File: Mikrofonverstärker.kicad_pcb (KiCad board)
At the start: 2 copper layers, 50.5 x 37.3 mm, 60 parts, among them J1 Screw_Terminal_01x02, J3 Screw_Terminal_01x02, J4 Screw_Terminal_01x03, J5 USB_C_Receptacle_USB2.0_14P, U1 CM108B, U2 THAT151xx08, U3 NMA0515SC

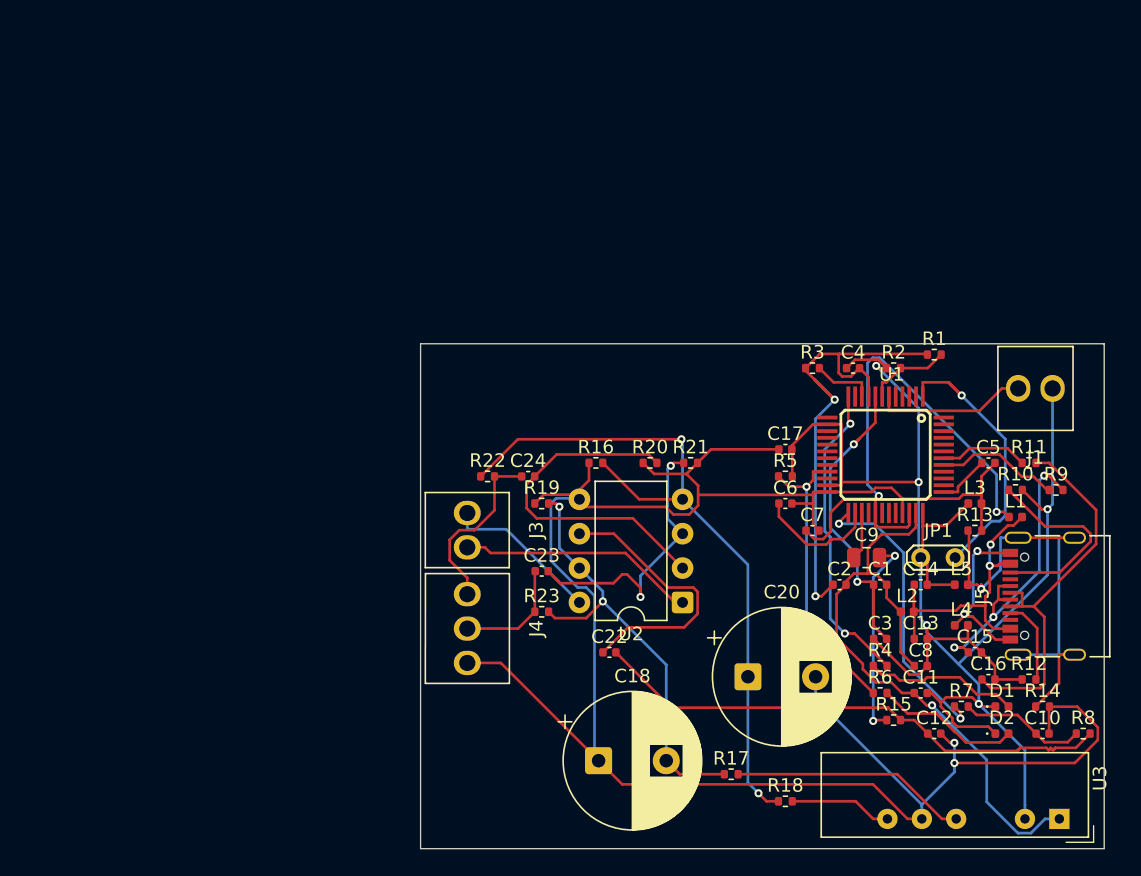
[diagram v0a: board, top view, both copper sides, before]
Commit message: schaltung ist fertig maschalla
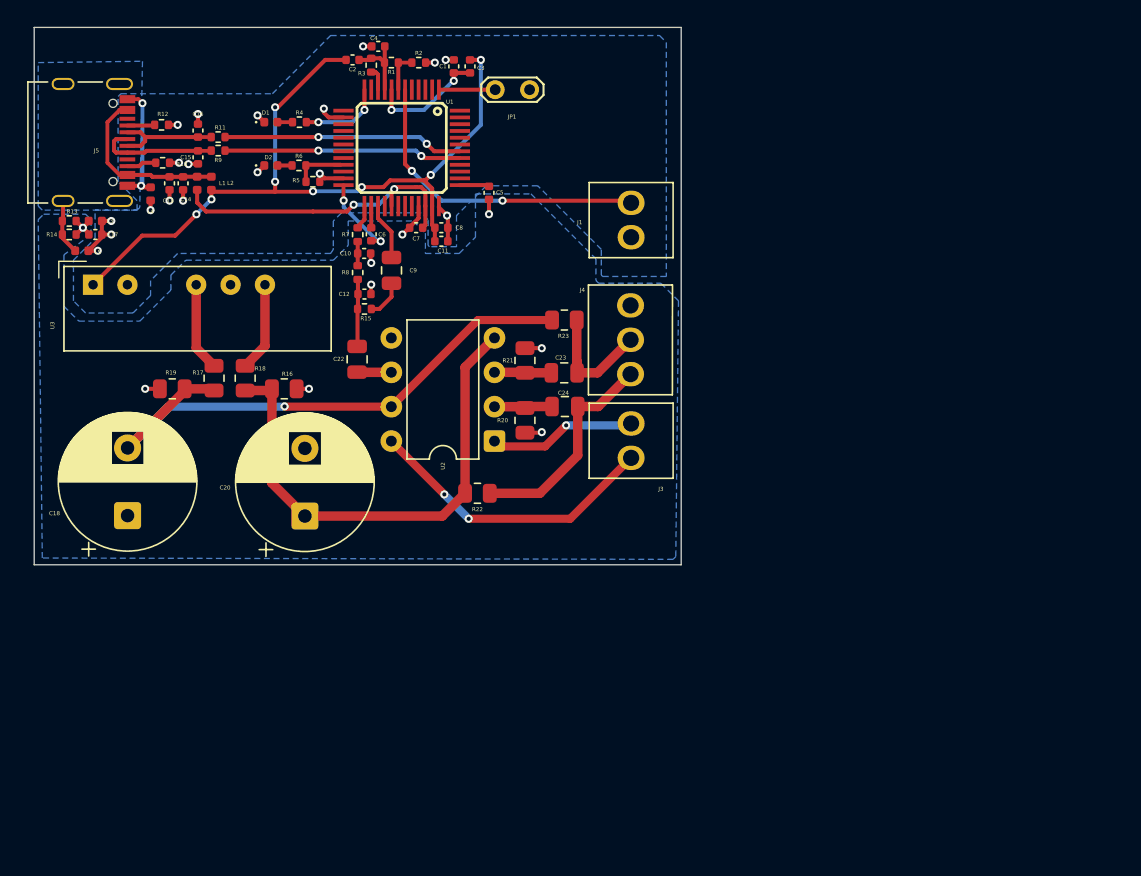
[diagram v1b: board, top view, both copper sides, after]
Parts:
- C22, C23, C24: footprint Capacitor_SMD:C_0402_1005Metric -> Capacitor_SMD:C_0805_2012Metric
- R16, R17, R18, R19, R20, R21, R22, R23: footprint Resistor_SMD:R_0402_1005Metric -> Resistor_SMD:R_0805_2012Metric
- moved U3 81.6 mm to (147.6, 100.0), turned to 90 degrees
- moved R14 79.9 mm to (145.8, 96.3)
- moved J5 77.8 mm to (147.6, 89.5), turned to -90 degrees
- moved R12 76.1 mm to (152.6, 88.2), turned to 180 degrees
- moved C16 71.1 mm to (155.3, 88.6), turned to 90 degrees
- moved R13 70.7 mm to (145.8, 95.3)
- moved L5 69.5 mm to (146.7, 97.5), turned to 180 degrees
- moved D1 69.1 mm to (160.7, 88.0)
- moved D2 68.4 mm to (160.7, 91.2)
- moved L3 68.3 mm to (147.7, 95.3), turned to 180 degrees
- moved C15 68.1 mm to (155.3, 90.6), turned to -90 degrees
- moved L4 67.8 mm to (151.8, 93.3), turned to -90 degrees
- moved R10 67.5 mm to (152.7, 91.0)
- moved R9 66.8 mm to (156.8, 90.1), turned to 180 degrees
- moved L1 65.3 mm to (155.2, 92.5), turned to 90 degrees
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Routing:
- net GNDA: track 162.9 -> 18.8 mm, vias 2 -> 11
- net GNDD: track 126.8 -> 20.6 mm, vias 5 -> 18
- net Net-(C2-Pad1): track 43.5 -> 5.21 mm, vias 2 -> 0
- net AMICIN: track 39.5 -> 4.85 mm
- net GNDPWR: track 35.9 -> 4.65 mm, vias 1 -> 0
- net Net-(U2--In): track 25.9 -> 4.34 mm
- net Net-(C16-Pad1): track 29.6 -> 8.10 mm
- net Net-(JP1-B): track 25.0 -> 4.16 mm, vias 1 -> 0
- net Net-(R7-Pad1): track 21.8 -> 1.81 mm, vias 2 -> 0
- net Net-(R5-Pad1): track 22.0 -> 3.80 mm, vias 2 -> 0
- net Net-(U2-Out): track 20.3 -> 2.62 mm
- net VAA: track 40.6 -> 23.1 mm
- net Net-(R4-Pad2): track 23.4 -> 6.17 mm
- net Net-(U2-+In): track 21.1 -> 4.22 mm, vias 2 -> 0
- net Net-(U2-V-): track 53.2 -> 37.3 mm, vias 2 -> 0
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- added copper zone on B.Cu, net GNDA
- added copper zone on B.Cu, net GNDD
- added copper zone on B.Cu, net GNDPWR
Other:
- board size 50.5 x 37.3 mm -> 47.8 x 39.7 mm
